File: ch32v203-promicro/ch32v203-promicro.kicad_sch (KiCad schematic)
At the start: 27 parts, among them J1 USB2.0_C_v3, J2 ProMicro-LeftPin, J3 ProMicro-RightPin, SW1 SW_Push, SW2 SW_Push, U1 CH32V203CxT6, U2 AMS1117-3.3, Y1 32.768k, Y2 8M

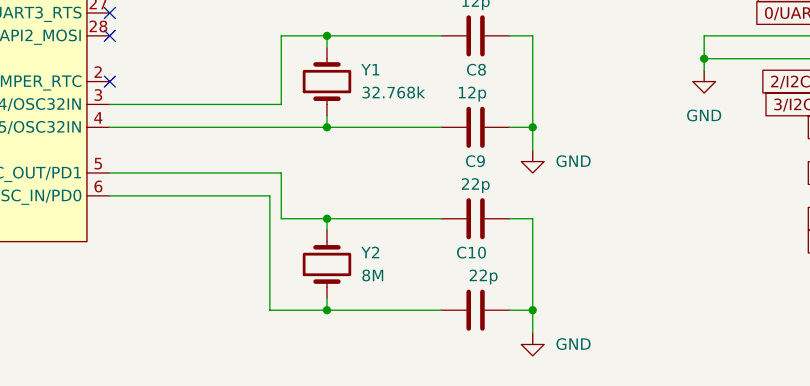
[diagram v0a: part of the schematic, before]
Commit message: wip
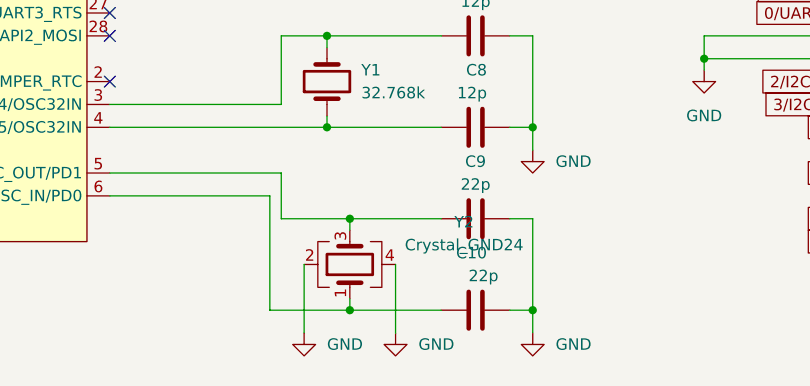
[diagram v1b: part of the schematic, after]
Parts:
- removed Y2: 8M, $74th:Crystal_SMD_3225-4Pin_3.2x2.5mm_HandSoldering, symbol Device:Crystal
- added Y2: Crystal_GND24, $74th:Crystal_SMD_3225-4Pin_3.2x2.5mm_HandSoldering, symbol Device:Crystal_GND24
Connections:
- net GND: now also Y2.2, Y2.4
- net at C10.1, U1.6 (OSC_IN/PD0): now also Y2.1
- net at C9.1, U1.5 (OSC_OUT/PD1): now also Y2.3
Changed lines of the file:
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@@
   (junction (at 250.19 36.83) (diameter 0) (color 0 0 0 0)
   )
-  (junction (at 157.48 132.08) (diameter 0) (color 0 0 0 0)
+  (junction (at 160.02 121.92) (diameter 0) (color 0 0 0 0)
   )
   (junction (at 113.03 25.4) (diameter 0) (color 0 0 0 0)
   )
-  (junction (at 157.48 121.92) (diameter 0) (color 0 0 0 0)
-  )
   (junction (at 157.48 111.76) (diameter 0) (color 0 0 0 0)
   )
@@
   )
   (junction (at 100.33 129.54) (diameter 0) (color 0 0 0 0)
+  )
+  (junction (at 160.02 132.08) (diameter 0) (color 0 0 0 0)
   )
   (junction (at 63.5 63.5) (diameter 0) (color 0 0 0 0)
@@
     (stroke (width 0) (type default) (color 0 0 0 0))
   )
-  (wire (pts (xy 157.48 130.81) (xy 157.48 132.08))
-    (stroke (width 0) (type default) (color 0 0 0 0))
-  )
   (wire (pts (xy 63.5 60.96) (xy 63.5 63.5))
     (stroke (width 0) (type default) (color 0 0 0 0))
   )
-  (wire (pts (xy 152.4 121.92) (xy 157.48 121.92))
-    (stroke (width 0) (type default) (color 0 0 0 0))
-  )
   (wire (pts (xy 199.39 101.6) (xy 199.39 104.14))
     (stroke (width 0) (type default) (color 0 0 0 0))
@@
     (stroke (width 0) (type default) (color 0 0 0 0))
   )
+  (wire (pts (xy 160.02 130.81) (xy 160.02 132.08))
+    (stroke (width 0) (type default) (color 0 0 0 0))
+  )
   (wire (pts (xy 217.17 55.88) (xy 217.17 57.15))
     (stroke (width 0) (type default) (color 0 0 0 0))
@@
     (stroke (width 0) (type default) (color 0 0 0 0))
   )
+  (wire (pts (xy 160.02 121.92) (xy 170.18 121.92))
+    (stroke (width 0) (type default) (color 0 0 0 0))
+  )
+  (wire (pts (xy 165.1 127) (xy 165.1 134.62))
+    (stroke (width 0) (type default) (color 0 0 0 0))
+  )
   (wire (pts (xy 180.34 101.6) (xy 177.8 101.6))
     (stroke (width 0) (type default) (color 0 0 0 0))
   )
+  (wire (pts (xy 154.94 127) (xy 154.94 134.62))
+    (stroke (width 0) (type default) (color 0 0 0 0))
+  )
   (wire (pts (xy 100.33 127) (xy 100.33 129.54))
     (stroke (width 0) (type default) (color 0 0 0 0))
@@
     (stroke (width 0) (type default) (color 0 0 0 0))
   )
-  (wire (pts (xy 157.48 132.08) (xy 170.18 132.08))
-    (stroke (width 0) (type default) (color 0 0 0 0))
-  )
-  (wire (pts (xy 157.48 123.19) (xy 157.48 121.92))
+  (wire (pts (xy 151.13 132.08) (xy 160.02 132.08))
     (stroke (width 0) (type default) (color 0 0 0 0))
   )
@@
     (stroke (width 0) (type default) (color 0 0 0 0))
   )
+  (wire (pts (xy 160.02 121.92) (xy 160.02 123.19))
+    (stroke (width 0) (type default) (color 0 0 0 0))
+  )
   (wire (pts (xy 44.45 68.58) (xy 64.77 68.58))
     (stroke (width 0) (type default) (color 0 0 0 0))
@@
     (stroke (width 0) (type default) (color 0 0 0 0))
   )
+  (wire (pts (xy 160.02 132.08) (xy 170.18 132.08))
+    (stroke (width 0) (type default) (color 0 0 0 0))
+  )
   (wire (pts (xy 113.03 25.4) (xy 125.73 25.4))
     (stroke (width 0) (type default) (color 0 0 0 0))
@@
     (stroke (width 0) (type default) (color 0 0 0 0))
   )
-  (wire (pts (xy 151.13 132.08) (xy 157.48 132.08))
-    (stroke (width 0) (type default) (color 0 0 0 0))
-  )
   (wire (pts (xy 16.51 59.69) (xy 16.51 58.42))
     (stroke (width 0) (type default) (color 0 0 0 0))
@@
     (stroke (width 0) (type default) (color 0 0 0 0))
   )
-  (wire (pts (xy 157.48 121.92) (xy 170.18 121.92))
+  (wire (pts (xy 152.4 121.92) (xy 160.02 121.92))
     (stroke (width 0) (type default) (color 0 0 0 0))
   )
@@
     )
     (property "Datasheet" "" (id 3) (at 237.49 44.45 0)
+      (effects (font (size 1.27 1.27)) hide)
+    )
+    (pin "1")
+  )
+  (symbol (lib_id "power:GND") (at 165.1 134.62 0) (unit 1)
+    (in_bom yes) (on_board yes) (fields_autoplaced)
+    (property "Reference" "#PWR0126" (id 0) (at 165.1 140.97 0)
+      (effects (font (size 1.27 1.27)) hide)
+    )
+    (property "Value" "GND" (id 1) (at 167.64 135.8899 0)
+      (effects (font (size 1.27 1.27)) (justify left))
+    )
+    (property "Footprint" "" (id 2) (at 165.1 134.62 0)
+      (effects (font (size 1.27 1.27)) hide)
+    )
+    (property "Datasheet" "" (id 3) (at 165.1 134.62 0)
       (effects (font (size 1.27 1.27)) hide)
     )
@@
     (pin "2")
     (pin "3")
-  )
-  (symbol (lib_id "Device:Crystal") (at 157.48 127 90) (unit 1)
-    (in_bom yes) (on_board yes) (fields_autoplaced)
-    (property "Reference" "Y2" (id 0) (at 161.29 125.7299 90)
-      (effects (font (size 1.27 1.27)) (justify right))
-    )
-    (property "Value" "8M" (id 1) (at 161.29 128.2699 90)
-      (effects (font (size 1.27 1.27)) (justify right))
-    )
-    (property "Footprint" "$74th:Crystal_SMD_3225-4Pin_3.2x2.5mm_HandSoldering" (id 2) (at 157.48 127 0)
-      (effects (font (size 1.27 1.27)) hide)
-    )
-    (property "Datasheet" "~" (id 3) (at 157.48 127 0)
-      (effects (font (size 1.27 1.27)) hide)
-    )
-    (pin "1")
-    (pin "2")
   )
   (symbol (lib_id "power:+3V3") (at 104.14 46.99 0) (unit 1)
@@
     (pin "1")
   )
+  (symbol (lib_id "Device:Crystal_GND24") (at 160.02 127 90) (unit 1)
+    (in_bom yes) (on_board yes) (fields_autoplaced)
+    (property "Reference" "Y2" (id 0) (at 172.72 122.301 90))
+    (property "Value" "Crystal_GND24" (id 1) (at 172.72 124.841 90))
+    (property "Footprint" "$74th:Crystal_SMD_3225-4Pin_3.2x2.5mm_HandSoldering" (id 2) (at 160.02 127 0)
+      (effects (font (size 1.27 1.27)) hide)
+    )
+    (property "Datasheet" "~" (id 3) (at 160.02 127 0)
+      (effects (font (size 1.27 1.27)) hide)
+    )
+    (pin "1")
+    (pin "2")
+    (pin "3")
+    (pin "4")
+  )
   (symbol (lib_id "Device:R") (at 228.6 60.96 0) (unit 1)
     (in_bom yes) (on_board yes) (fields_autoplaced)
@@
     (pin "1")
   )
+  (symbol (lib_id "power:GND") (at 154.94 134.62 0) (unit 1)
+    (in_bom yes) (on_board yes) (fields_autoplaced)
+    (property "Reference" "#PWR0127" (id 0) (at 154.94 140.97 0)
+      (effects (font (size 1.27 1.27)) hide)
+    )
+    (property "Value" "GND" (id 1) (at 157.48 135.8899 0)
+      (effects (font (size 1.27 1.27)) (justify left))
+    )
+    (property "Footprint" "" (id 2) (at 154.94 134.62 0)
+      (effects (font (size 1.27 1.27)) hide)
+    )
+    (property "Datasheet" "" (id 3) (at 154.94 134.62 0)
+      (effects (font (size 1.27 1.27)) hide)
+    )
+    (pin "1")
+  )
   (symbol (lib_id "Device:R") (at 217.17 60.96 0) (unit 1)
     (in_bom yes) (on_board yes) (fields_autoplaced)
@@
       (reference "#PWR0125") (unit 1) (value "GND") (footprint "")
     )
+    (path "/1e6bbce5-22a4-413a-ae6c-9674ee0ec340"
+      (reference "#PWR0126") (unit 1) (value "GND") (footprint "")
+    )
+    (path "/f7161deb-d265-4803-ab6d-3576c1d8028a"
+      (reference "#PWR0127") (unit 1) (value "GND") (footprint "")
+    )
     (path "/14ed74d4-0c4d-4835-b05c-faed62dadd13"
       (reference "C1") (unit 1) (value "100n") (footprint "$74th:Capacitor_0805_2012")
@@
       (reference "Y1") (unit 1) (value "32.768k") (footprint "Crystal:Crystal_SMD_3215-2Pin_3.2x1.5mm")
     )
-    (path "/9dfaf330-cc68-412b-b211-e02aaa69f0bf"
-      (reference "Y2") (unit 1) (value "8M") (footprint "$74th:Crystal_SMD_3225-4Pin_3.2x2.5mm_HandSoldering")
-    )
-  )
+    (path "/c74f931d-165a-4d8e-ac35-db57a47886df"
+      (reference "Y2") (unit 1) (value "Crystal_GND24") (footprint "$74th:Crystal_SMD_3225-4Pin_3.2x2.5mm_HandSoldering")
+    )
+  )

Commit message: ch32v203 promicro
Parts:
- J2: footprint Connector_PinHeader_2.54mm:PinHeader_1x12_P2.54mm_Vertical -> $74th:ProMicro_LIKE_LEFT
- J3: footprint Connector_PinHeader_2.54mm:PinHeader_1x12_P2.54mm_Vertical -> $74th:ProMicro_LIKE_RIGHT
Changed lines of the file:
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@@
     (property "Reference" "J2" (id 0) (at 224.155 90.17 0))
     (property "Value" "ProMicro-LeftPin" (id 1) (at 224.155 92.71 0))
-    (property "Footprint" "Connector_PinHeader_2.54mm:PinHeader_1x12_P2.54mm_Vertical" (id 2) (at 223.52 93.98 0)
+    (property "Footprint" "$74th:ProMicro_LIKE_LEFT" (id 2) (at 223.52 93.98 0)
       (effects (font (size 1.27 1.27)) hide)
     )
@@
     (property "Reference" "J3" (id 0) (at 252.095 91.44 0))
     (property "Value" "ProMicro-RightPin" (id 1) (at 252.095 93.98 0))
-    (property "Footprint" "Connector_PinHeader_2.54mm:PinHeader_1x12_P2.54mm_Vertical" (id 2) (at 248.92 95.25 0)
+    (property "Footprint" "$74th:ProMicro_LIKE_RIGHT" (id 2) (at 248.92 95.25 0)
       (effects (font (size 1.27 1.27)) hide)
     )
@@
     )
     (path "/7375c197-3897-4432-8938-1ae5a4f6e3d0"
-      (reference "J2") (unit 1) (value "ProMicro-LeftPin") (footprint "Connector_PinHeader_2.54mm:PinHeader_1x12_P2.54mm_Vertical")
+      (reference "J2") (unit 1) (value "ProMicro-LeftPin") (footprint "$74th:ProMicro_LIKE_LEFT")
     )
     (path "/e1e03df2-7a42-4865-baeb-e2d3f6f87dbd"
-      (reference "J3") (unit 1) (value "ProMicro-RightPin") (footprint "Connector_PinHeader_2.54mm:PinHeader_1x12_P2.54mm_Vertical")
+      (reference "J3") (unit 1) (value "ProMicro-RightPin") (footprint "$74th:ProMicro_LIKE_RIGHT")
     )
     (path "/147c7672-da6d-4d35-b258-1722de507206"

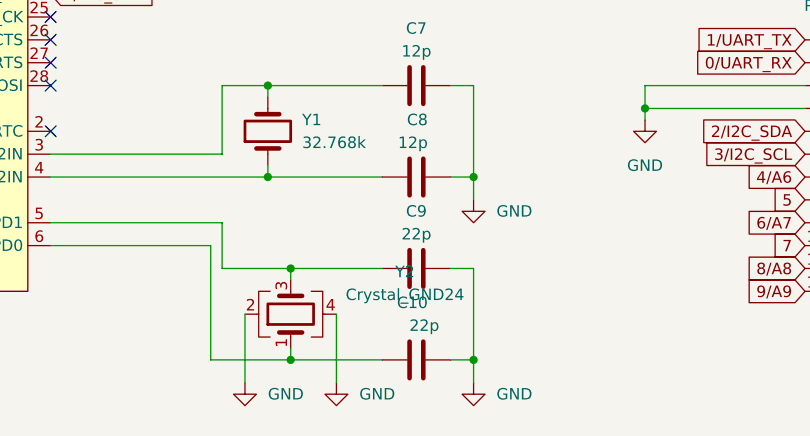
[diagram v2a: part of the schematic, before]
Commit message: ch32v203micro
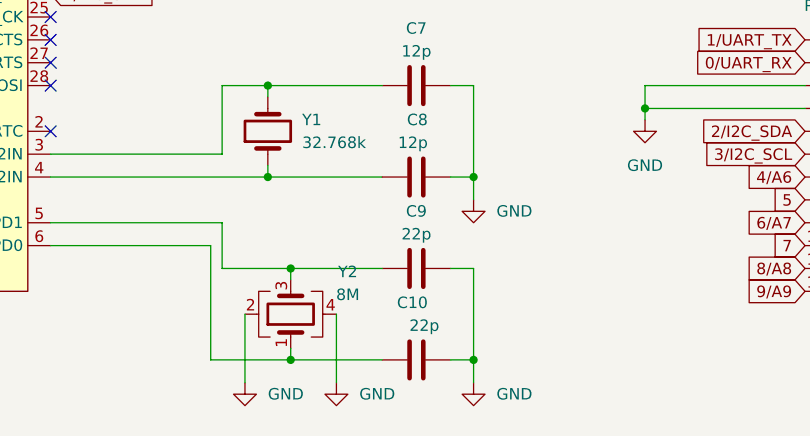
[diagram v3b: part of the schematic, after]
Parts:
- Y1: footprint Crystal:Crystal_SMD_3215-2Pin_3.2x1.5mm -> $74th:Crystal_SMD_3215-2Pin_3.2x1.5mm
- Y2: value Crystal_GND24 -> 8M
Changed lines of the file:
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@@
   (symbol (lib_id "Device:Crystal_GND24") (at 160.02 127 90) (unit 1)
     (in_bom yes) (on_board yes) (fields_autoplaced)
-    (property "Reference" "Y2" (id 0) (at 172.72 122.301 90))
-    (property "Value" "Crystal_GND24" (id 1) (at 172.72 124.841 90))
+    (property "Reference" "Y2" (id 0) (at 166.37 122.301 90))
+    (property "Value" "8M" (id 1) (at 166.37 124.841 90))
     (property "Footprint" "$74th:Crystal_SMD_3225-4Pin_3.2x2.5mm_HandSoldering" (id 2) (at 160.02 127 0)
       (effects (font (size 1.27 1.27)) hide)
@@
       (effects (font (size 1.27 1.27)) (justify right))
     )
-    (property "Footprint" "Crystal:Crystal_SMD_3215-2Pin_3.2x1.5mm" (id 2) (at 157.48 106.68 0)
+    (property "Footprint" "$74th:Crystal_SMD_3215-2Pin_3.2x1.5mm" (id 2) (at 157.48 106.68 0)
       (effects (font (size 1.27 1.27)) hide)
     )
@@
     )
     (path "/e571ffa6-16f7-40af-86a7-417e167da2f9"
-      (reference "Y1") (unit 1) (value "32.768k") (footprint "Crystal:Crystal_SMD_3215-2Pin_3.2x1.5mm")
+      (reference "Y1") (unit 1) (value "32.768k") (footprint "$74th:Crystal_SMD_3215-2Pin_3.2x1.5mm")
     )
     (path "/c74f931d-165a-4d8e-ac35-db57a47886df"
-      (reference "Y2") (unit 1) (value "Crystal_GND24") (footprint "$74th:Crystal_SMD_3225-4Pin_3.2x2.5mm_HandSoldering")
-    )
-  )
+      (reference "Y2") (unit 1) (value "8M") (footprint "$74th:Crystal_SMD_3225-4Pin_3.2x2.5mm_HandSoldering")
+    )
+  )

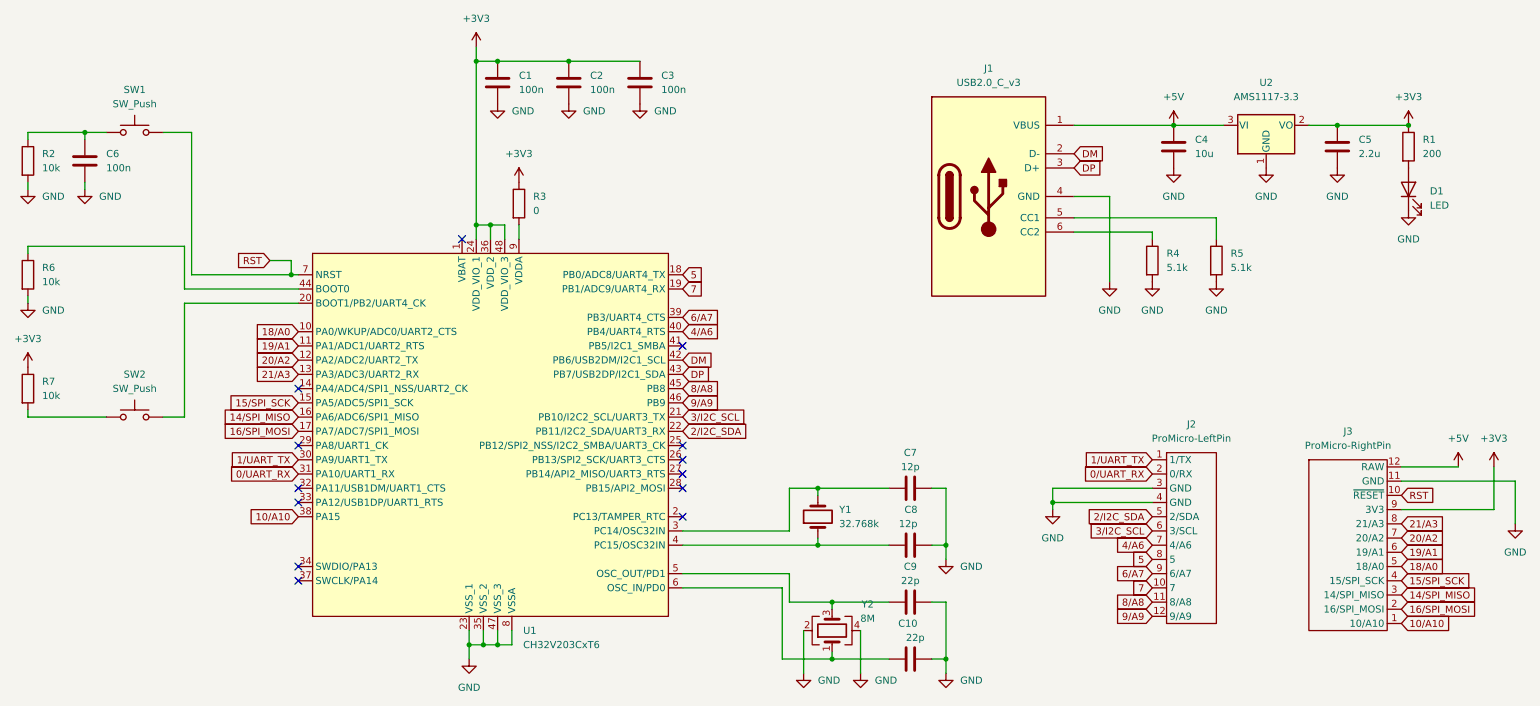
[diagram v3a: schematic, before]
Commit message: ch32v203micro v1.0.0
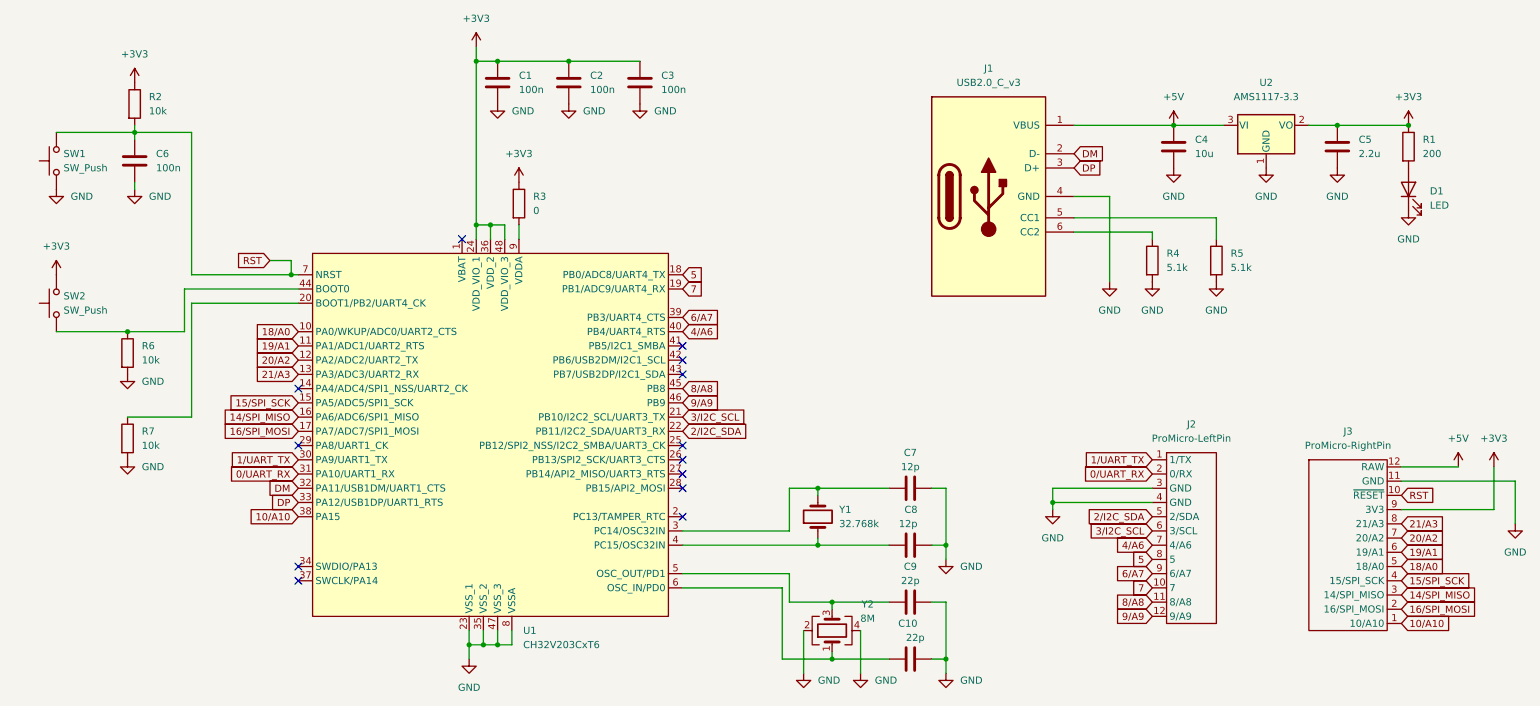
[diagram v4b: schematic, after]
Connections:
- net +3V3: now also R2.1, SW2.2; no longer R7.1
- net DM: now also U1.32 (PA11/USB1DM/UART1_CTS); no longer U1.42 (PB6/USB2DM/I2C1_SCL)
- net DP: now also U1.33 (PA12/USB1DP/UART1_RTS); no longer U1.43 (PB7/USB2DP/I2C1_SDA)
- net GND: now also R7.2, SW1.1; no longer R2.2
- net RST: now also C6.1, R2.2
- net at R6.1, U1.44 (BOOT0): now also SW2.1
- net at U1.20 (BOOT1/PB2/UART4_CK): now also R7.1; no longer SW2.2
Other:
- moved on the sheet: C6, R6, R7, SW1, SW2
